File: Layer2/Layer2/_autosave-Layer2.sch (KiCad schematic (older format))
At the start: 34 parts, among them J1 Conn_02x20_Odd_Even, J2 Conn_02x20_Odd_Even, U1 74LS08, U10 74HC245, U11 74HC245, U12 74LS181, U13 28C256, U14 74LS173, U15 628128_DIP32_SSOP32, U16 74LS173, U17 74LS85, U18 74LS08, U19 74LS273, U2 74HC273, U20 74LS273, U3 74HC273, U4 74HC273, U5 74HC245, U6 74HC245, U7 74HC245, U8 74LS181, U9 74HC273

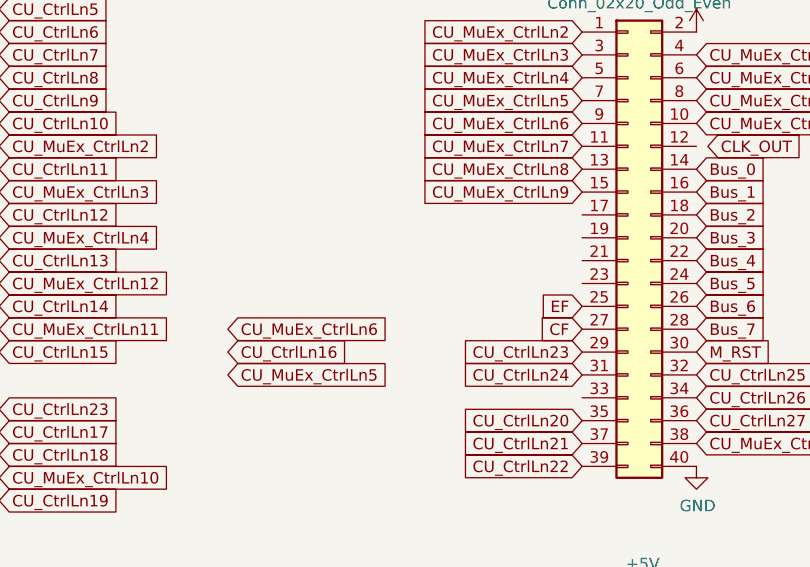
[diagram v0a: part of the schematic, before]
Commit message: Layer 3 complete
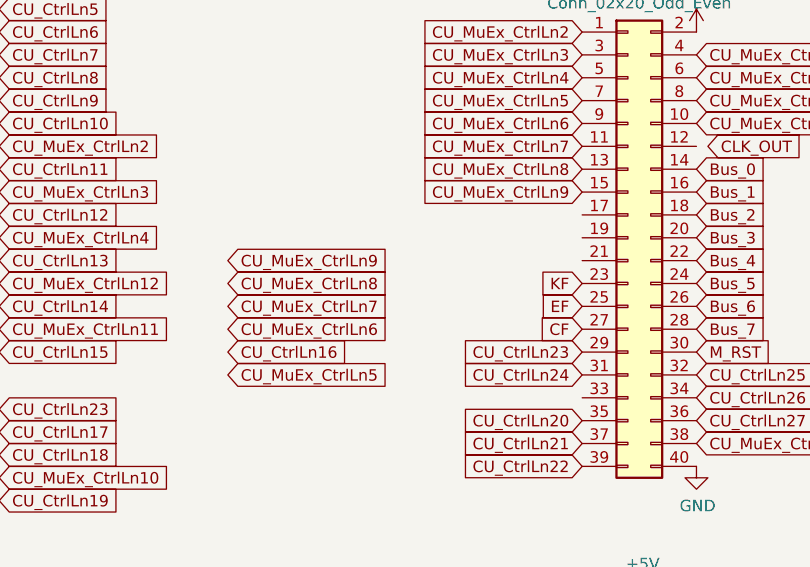
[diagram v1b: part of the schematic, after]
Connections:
- net KF: now reaches J2.23 (Pin_23)
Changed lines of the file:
@@
 $EndComp
 Connection ~ 5800 10150
+Text GLabel 8300 4400 2    50   Input ~ 0
+CU_MuEx_CtrlLn7
+Text GLabel 8300 4300 2    50   Input ~ 0
+CU_MuEx_CtrlLn8
+Text GLabel 8300 4200 2    50   Input ~ 0
+CU_MuEx_CtrlLn9
+Text GLabel 9850 4300 0    50   Input ~ 0
+KF
 $EndSCHEMATC
